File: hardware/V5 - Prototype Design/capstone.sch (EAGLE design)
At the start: 25 parts, among them U1 ADAFRUIT_MPL3115A2_BAROMETER, U2 ADAFRUIT_MTK3339_GPS, U4 SPARKFUN_MPU9250_IMU, U5 RFM95W-915S2

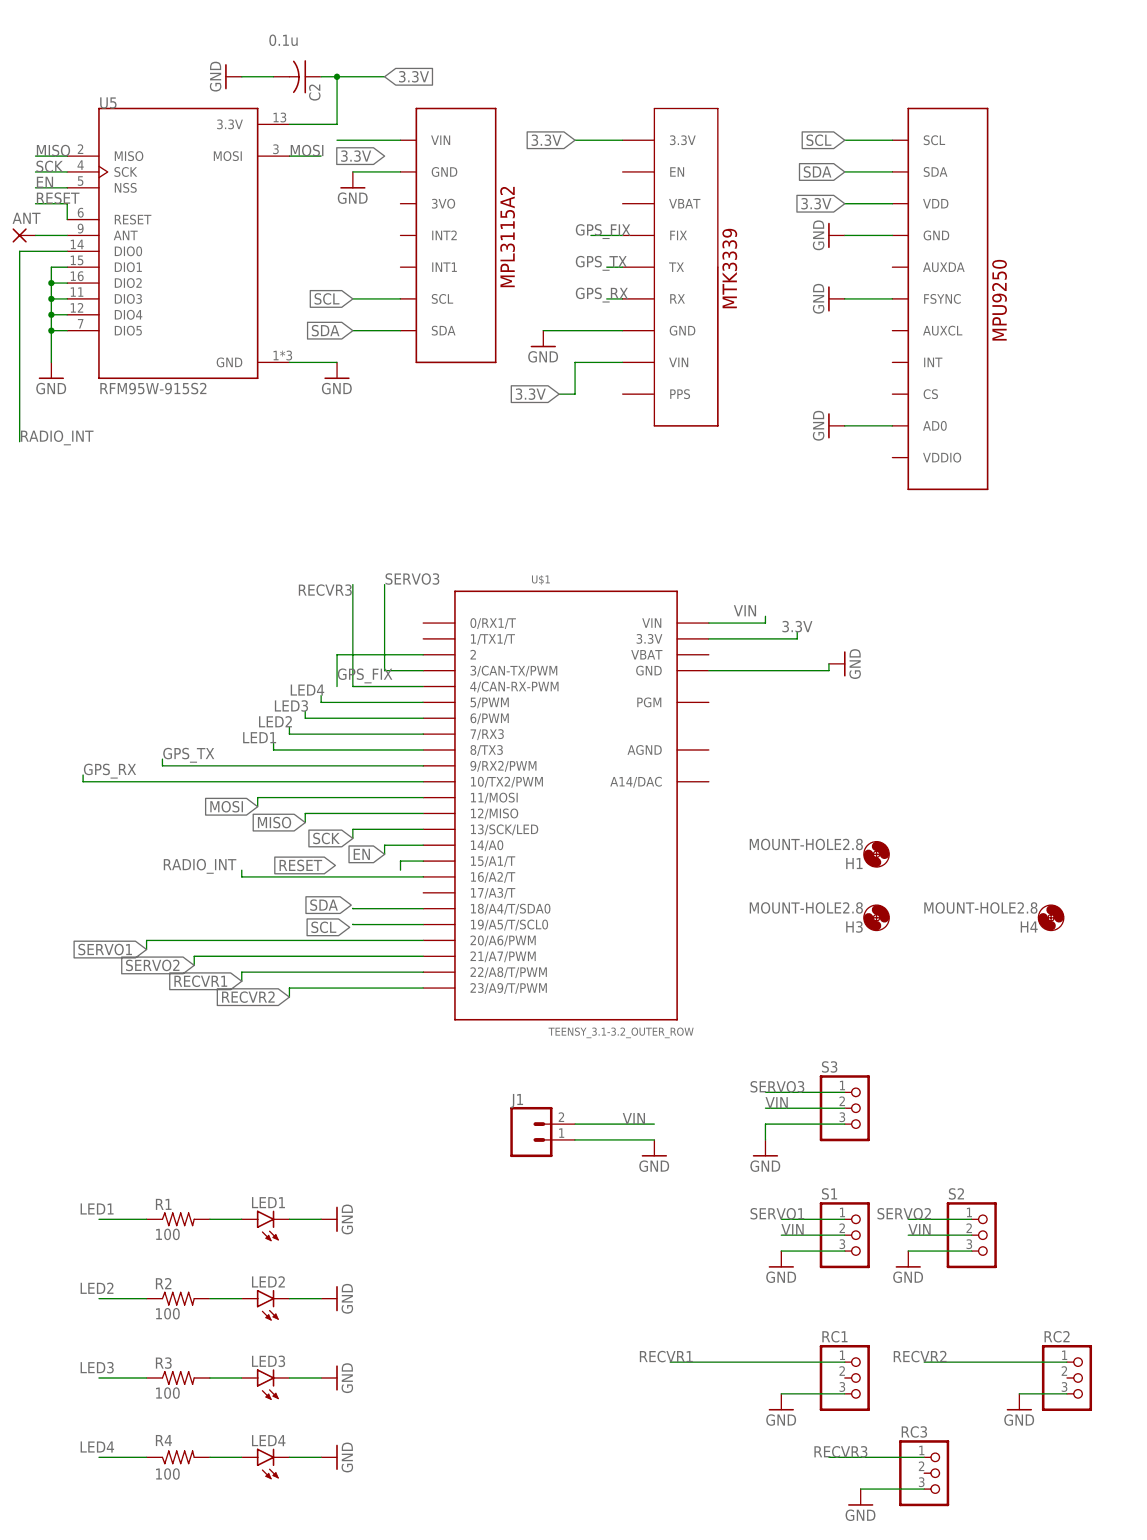
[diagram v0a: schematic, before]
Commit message: Schematic Cleanup
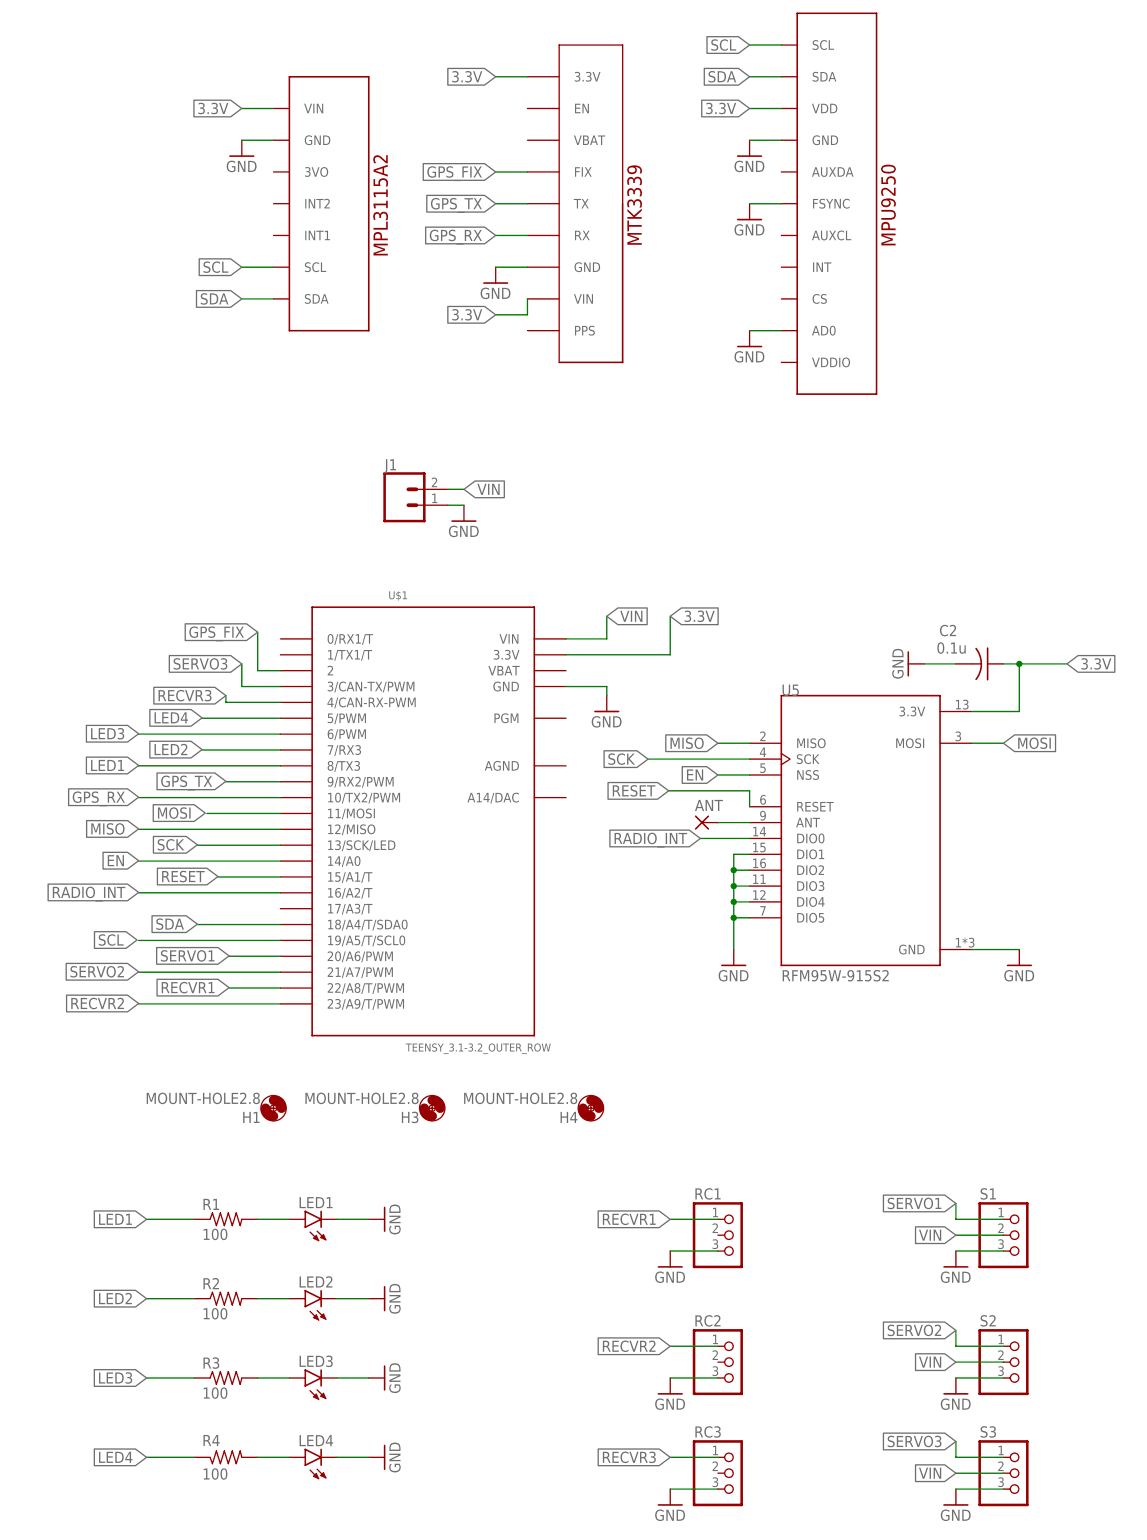
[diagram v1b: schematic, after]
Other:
- note added: "Barometer"
- note added: "Battery Input"
- note added: "Debugging LEDs"
- note added: "GPS"
- note added: "IMU"
- note added: "Microcontroller"
- note added: "Mounting Holes"
- note added: "Radio"
- note added: "Receiver Inputs"
- note added: "Servo Outputs"
- moved on the sheet: ANT, C2, H1, H3, H4, J1, LED1, LED2, LED3, LED4, R1, R2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
